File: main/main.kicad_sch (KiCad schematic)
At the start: 72 parts, among them J1 Conn_01x03, J10 Conn_01x02, J11 Conn_01x02, J12 Conn_01x02, J13 Conn_01x02, J14 Conn_01x02, J15 Conn_01x02, J16 Conn_01x02, J17 Conn_01x02, J18 Conn_01x02, J19 Conn_01x02, J2 Conn_01x03, J20 Conn_01x04, J21 Conn_01x04, J22 Conn_01x06, J23 Conn_01x03, J24 Conn_01x06_Pin, J3 Conn_01x03, J4 Conn_01x03, J5 Conn_01x03, J6 Conn_01x03, J7 Conn_01x03, J8 Conn_01x03, J9 Conn_01x02, SW1 SW_DIP_x01, SW2 SW_DIP_x01, U1 XT30U-F, U2 ESP32-S3-WROOM-1, U8 CH340N, U9 AMS1117-3.3, X1 32.768KHz

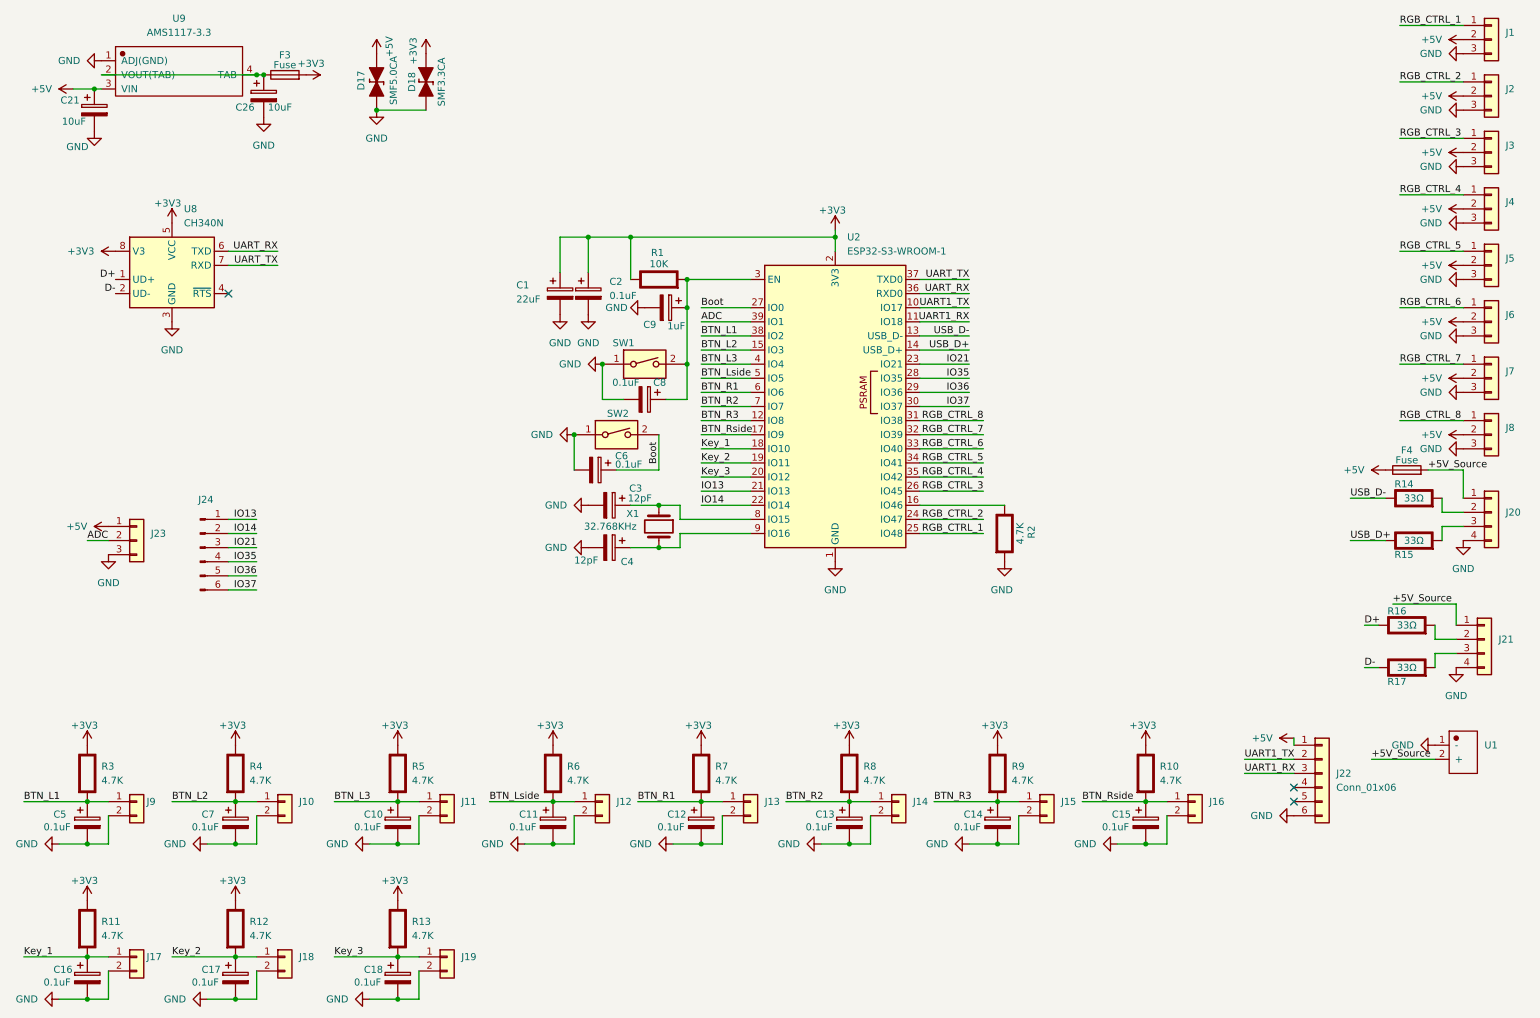
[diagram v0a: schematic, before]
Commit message: V1.1
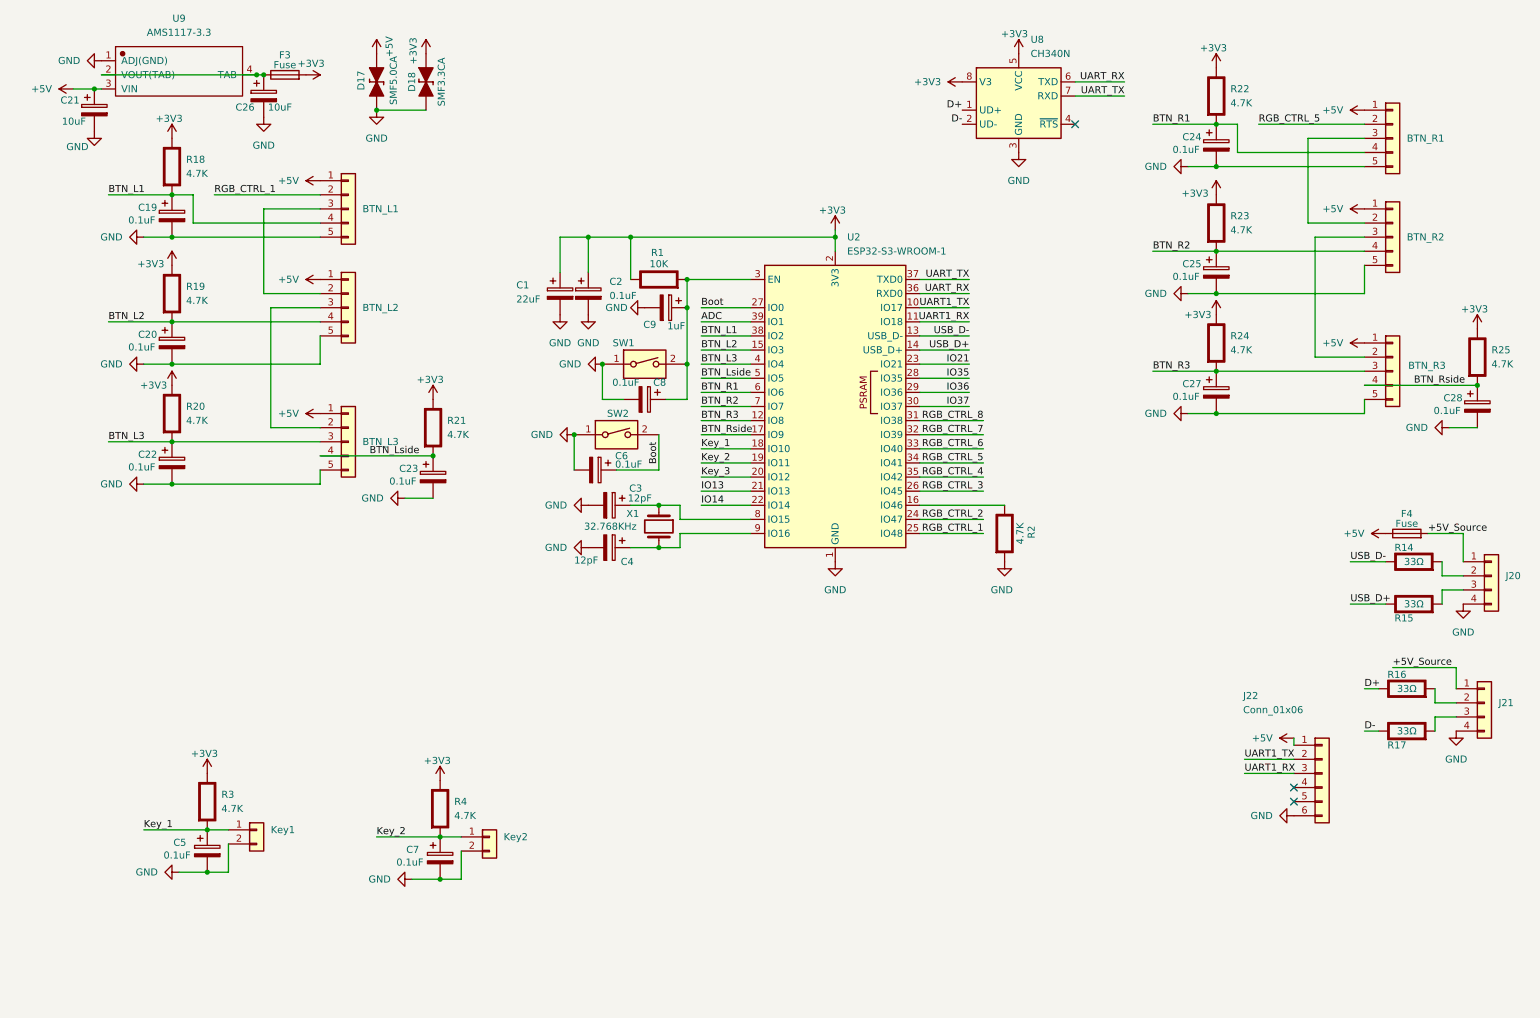
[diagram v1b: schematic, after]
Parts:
- removed C10, C11, C12, C13, C14, C15, C16, C17, C18: 0.1uF, Capacitor_SMD:C_0603_1608Metric_Pad1.08x0.95mm_HandSolder, symbol Device:C_Polarized
- removed J1, J2, J3, J4, J5, J6, J7, J8: Conn_01x03, Connector:FanPinHeader_1x03_P2.54mm_Vertical, symbol Connector_Generic:Conn_01x03
- removed J10, J11, J12, J13, J14, J15, J16, J17, J18, J19, J9: Conn_01x02, Connector_JST:JST_SH_BM02B-SRSS-TB_1x02-1MP_P1.00mm_Vertical, symbol Connector_Generic:Conn_01x02
- removed J23: Conn_01x03, Connector_JST:JST_SH_BM03B-SRSS-TB_1x03-1MP_P1.00mm_Vertical, symbol Connector_Generic:Conn_01x03
- removed J24: Conn_01x06_Pin, Connector_PinHeader_2.54mm:PinHeader_1x06_P2.54mm_Vertical, symbol Connector:Conn_01x06_Pin
- removed R10, R11, R12, R13, R5, R6, R7, R8, R9: 4.7K, Resistor_SMD:R_0805_2012Metric, symbol PCM_Elektuur:R
- removed U1: XT30U-F, XT:CONN-TH_XT30U-M, symbol XT:XT30U-F
- added BTN_L1, BTN_L2, BTN_L3, BTN_R1, BTN_R2, BTN_R3: Conn_01x05, Connector_JST:JST_XH_B5B-XH-AM_1x05_P2.50mm_Vertical, symbol Connector_Generic:Conn_01x05
- added C19, C20, C22, C23, C24, C25, C27, C28: 0.1uF, Capacitor_SMD:C_0603_1608Metric_Pad1.08x0.95mm_HandSolder, symbol Device:C_Polarized
- added Key1, Key2: Conn_01x02, Connector_JST:JST_XH_B2B-XH-AM_1x02_P2.50mm_Vertical, symbol Connector_Generic:Conn_01x02
- added R18, R19, R20, R21, R22, R23, R24, R25: 4.7K, Resistor_SMD:R_0805_2012Metric, symbol PCM_Elektuur:R
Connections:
- net +3V3: now also R18.1 (+), R19.1 (+), R20.1 (+), R21.1 (+), R22.1 (+), R23.1 (+), R24.1 (+), R25.1 (+)
- net +5V: now also BTN_L1.1 (Pin_1), BTN_L2.1 (Pin_1), BTN_L3.1 (Pin_1), BTN_R1.1 (Pin_1), BTN_R2.1 (Pin_1), BTN_R3.1 (Pin_1)
- net BTN_L1: now also BTN_L1.4 (Pin_4), C19.1, R18.2 (-); no longer C5.1, R3.2 (-)
- net BTN_L2: now also BTN_L2.4 (Pin_4), C20.1, R19.2 (-); no longer C7.1, R4.2 (-)
- net BTN_L3: now also BTN_L3.3 (Pin_3), C22.1, R20.2 (-)
- net BTN_Lside: now also BTN_L3.4 (Pin_4), C23.1, R21.2 (-)
- net BTN_R1: now also BTN_R1.4 (Pin_4), C24.1, R22.2 (-)
- net BTN_R2: now also BTN_R2.4 (Pin_4), C25.1, R23.2 (-)
- net BTN_R3: now also BTN_R3.3 (Pin_3), C27.1, R24.2 (-)
- net BTN_Rside: now also BTN_R3.4 (Pin_4), C28.1, R25.2 (-)
- net GND: now also BTN_L1.5 (Pin_5), BTN_L2.5 (Pin_5), BTN_L3.5 (Pin_5), BTN_R1.5 (Pin_5), BTN_R2.5 (Pin_5), BTN_R3.5 (Pin_5), C19.2, C20.2, C22.2, C23.2, C24.2, C25.2, C27.2, C28.2, Key1.2 (Pin_2), Key2.2 (Pin_2)
- net Key_1: now also C5.1, R3.2 (-), Key1.1 (Pin_1)
- net Key_2: now also C7.1, R4.2 (-), Key2.1 (Pin_1)
- net RGB_CTRL_1: now also BTN_L1.2 (Pin_2)
- net RGB_CTRL_5: now also BTN_R1.2 (Pin_2)
- new net: BTN_R1.3 (Pin_3), BTN_R2.2 (Pin_2)
- new net: BTN_L1.3 (Pin_3), BTN_L2.2 (Pin_2)
- new net: BTN_L2.3 (Pin_3), BTN_L3.2 (Pin_2)
- new net: BTN_R2.3 (Pin_3), BTN_R3.2 (Pin_2)
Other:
- moved on the sheet: F4, J20, J21, R14, R15, R16, R17, U8
